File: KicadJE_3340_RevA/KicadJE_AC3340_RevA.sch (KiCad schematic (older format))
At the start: 125 parts, among them J101 RampOut1, J102 PulseOut2, J103 SawOut3, J104 In1.1, J105 In1.2, J106 In1.3, J107 SS_In2, J108 HS_In3, J109 FM_In4, J110 PWM_In5, J111 SineOut4, P101 HEADER_2x5_Doepfer, Q101 MMBT3906, Q102 UMX1N, SW101 Octave (3 state), U101 TL072, U102 TL072, U103 TL072, U104 AS3340, U105 L78L05_SOT89, U106 L79L05_SOT89, U107 TL072

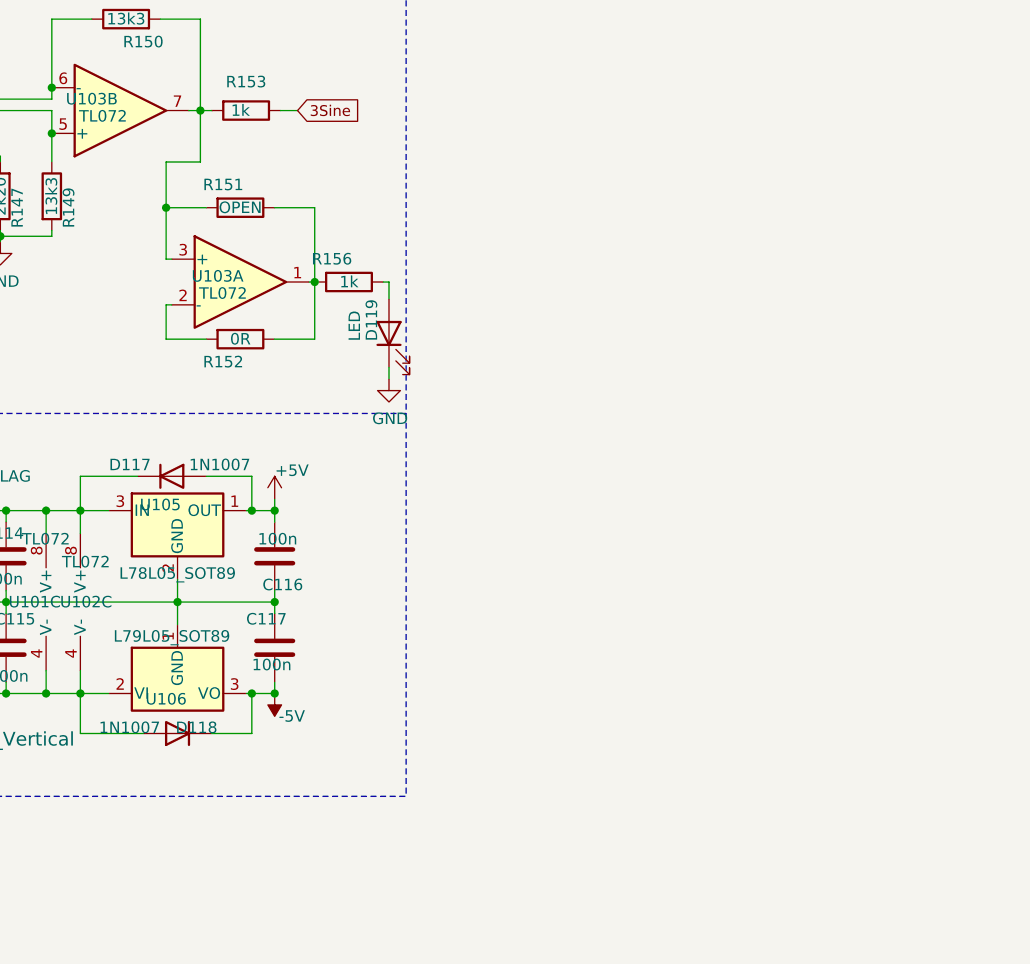
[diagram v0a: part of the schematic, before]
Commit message: Update KicadJE_AC3340_RevA.sch
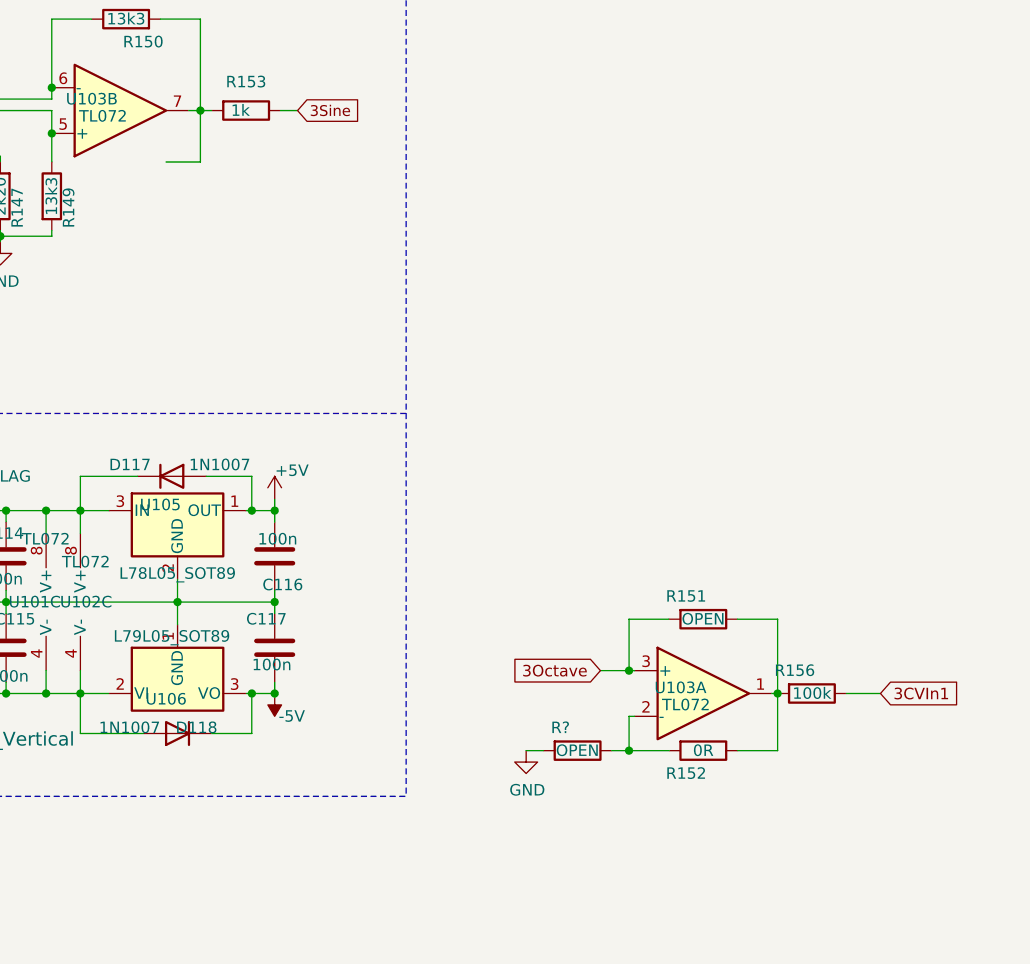
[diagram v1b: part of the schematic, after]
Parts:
- removed D119: LED, LED_SMD:LED_0805_2012Metric_Pad1.15x1.40mm_HandSolder, symbol Device:LED
- added R?: OPEN, Resistor_SMD:R_0805_2012Metric_Pad1.15x1.40mm_HandSolder, symbol Device:R
- R156: value 1k -> 100k
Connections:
- net 3CVIn1: now also R156.1
- net 3Octave: now also R151.2, U103.3 (+)
- net GND: now also R?.2
- net at R150.2, R153.2, U103.7: no longer R151.2, U103.3 (+)
- net at R152.2, U103.2 (-): now also R?.1
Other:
- moved on the sheet: R151, R152, R156, U103A
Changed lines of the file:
@@
 L Amplifier_Operational:TL072 U?
 U 1 1 614891B3
-P 7725 4275
+P 9750 6075
 AR Path="/5D99B81E/614891B3" Ref="U?"  Part="3"
 AR Path="/5D99B7BA/614891B3" Ref="U?"  Part="1"
@@
 AR Path="/5F49A670/614891B3" Ref="U?"  Part="1"
 AR Path="/614891B3" Ref="U103"  Part="1"
-F 0 "U103" H 7625 4300 50  0000 C CNN
-F 1 "TL072" H 7650 4225 50  0000 C CNN
-F 2 "AJ-Dropbox-Kicad:AJ_SO-8_5.3x6.2mm_P1.27mm" H 7725 4275 50  0001 C CNN
-F 3 "http://www.ti.com/lit/ds/symlink/tl071.pdf" H 7725 4275 50  0001 C CNN
-	1    7725 4275
+F 0 "U103" H 9650 6100 50  0000 C CNN
+F 1 "TL072" H 9675 6025 50  0000 C CNN
+F 2 "AJ-Dropbox-Kicad:AJ_SO-8_5.3x6.2mm_P1.27mm" H 9750 6075 50  0001 C CNN
+F 3 "http://www.ti.com/lit/ds/symlink/tl071.pdf" H 9750 6075 50  0001 C CNN
+	1    9750 6075
 	1    0    0    -1
 $EndComp
 Wire Wire Line
-	7425 4375 7400 4375
+	9450 6175 9425 6175
 Wire Wire Line
-	7400 4375 7400 4525
+	9425 6175 9425 6325
 Wire Wire Line
-	7400 4525 7575 4525
+	9425 6325 9600 6325
 Wire Wire Line
-	8050 4525 8050 4275
+	10075 6325 10075 6075
 Wire Wire Line
-	8050 4275 8025 4275
+	10075 6075 10050 6075
 $Comp
 L Device:R R156
 U 1 1 614891BF
-P 8200 4275
+P 10225 6075
 AR Path="/614891BF" Ref="R156"  Part="1"
 AR Path="/5C8C5FC0/614891BF" Ref="R?"  Part="1"
@@
 AR Path="/5E62ACA1/614891BF" Ref="R?"  Part="1"
 AR Path="/5F49A670/614891BF" Ref="R?"  Part="1"
-F 0 "R156" V 8100 4200 50  0000 C CNN
-F 1 "1k" V 8200 4275 50  0000 C CNN
-F 2 "Resistor_SMD:R_0805_2012Metric_Pad1.15x1.40mm_HandSolder" V 8130 4275 50  0001 C CNN
-F 3 "~" H 8200 4275 50  0001 C CNN
-	1    8200 4275
+F 0 "R156" V 10125 6000 50  0000 C CNN
+F 1 "100k" V 10225 6075 50  0000 C CNN
+F 2 "Resistor_SMD:R_0805_2012Metric_Pad1.15x1.40mm_HandSolder" V 10155 6075 50  0001 C CNN
+F 3 "~" H 10225 6075 50  0001 C CNN
+	1    10225 6075
 	0    1    1    0
 $EndComp
-Connection ~ 8050 4275
+Connection ~ 10075 6075
 Wire Wire Line
 	2400 1125 2325 1125
@@
 L Device:R R151
 U 1 1 61551447
-P 7725 3950
+P 9750 5750
 AR Path="/61551447" Ref="R151"  Part="1"
 AR Path="/5C8C5FC0/61551447" Ref="R?"  Part="1"
@@
 AR Path="/5E62ACA1/61551447" Ref="R?"  Part="1"
 AR Path="/5F49A670/61551447" Ref="R?"  Part="1"
-F 0 "R151" V 7625 3875 50  0000 C CNN
-F 1 "OPEN" V 7725 3950 50  0000 C CNN
-F 2 "Resistor_SMD:R_0805_2012Metric_Pad1.15x1.40mm_HandSolder" V 7655 3950 50  0001 C CNN
-F 3 "~" H 7725 3950 50  0001 C CNN
-	1    7725 3950
+F 0 "R151" V 9650 5675 50  0000 C CNN
+F 1 "OPEN" V 9750 5750 50  0000 C CNN
+F 2 "Resistor_SMD:R_0805_2012Metric_Pad1.15x1.40mm_HandSolder" V 9680 5750 50  0001 C CNN
+F 3 "~" H 9750 5750 50  0001 C CNN
+	1    9750 5750
 	0    1    1    0
 $EndComp
 Wire Wire Line
-	7400 4175 7400 3950
+	9425 5975 9425 5750
 Wire Wire Line
-	7400 3950 7575 3950
+	9425 5750 9600 5750
 Wire Wire Line
-	7400 4175 7425 4175
+	9425 5975 9450 5975
 Wire Wire Line
-	8050 4275 8050 3950
+	10075 6075 10075 5750
 Wire Wire Line
-	8050 3950 7875 3950
+	10075 5750 9900 5750
 $Comp
 L Envelope-cache-2018-08-04-13-00-04:GND #PWR0125
@@
 Wire Wire Line
 	7550 3750 7400 3750
-Wire Wire Line
-	7400 3750 7400 3950
-Connection ~ 7400 3950
 $Comp
 L Device:R R152
 U 1 1 616AB5FE
-P 7725 4525
+P 9750 6325
 AR Path="/616AB5FE" Ref="R152"  Part="1"
 AR Path="/5C8C5FC0/616AB5FE" Ref="R?"  Part="1"
@@
 AR Path="/5E62ACA1/616AB5FE" Ref="R?"  Part="1"
 AR Path="/5F49A670/616AB5FE" Ref="R?"  Part="1"
-F 0 "R152" V 7825 4450 50  0000 C CNN
-F 1 "0R" V 7725 4525 50  0000 C CNN
-F 2 "Resistor_SMD:R_0805_2012Metric_Pad1.15x1.40mm_HandSolder" V 7655 4525 50  0001 C CNN
-F 3 "~" H 7725 4525 50  0001 C CNN
-	1    7725 4525
+F 0 "R152" V 9850 6250 50  0000 C CNN
+F 1 "0R" V 9750 6325 50  0000 C CNN
+F 2 "Resistor_SMD:R_0805_2012Metric_Pad1.15x1.40mm_HandSolder" V 9680 6325 50  0001 C CNN
+F 3 "~" H 9750 6325 50  0001 C CNN
+	1    9750 6325
 	0    1    1    0
 $EndComp
 Wire Wire Line
-	7875 4525 8050 4525
+	9900 6325 10075 6325
+Text GLabel 10525 6075 2    50   Input ~ 0
+3CVIn1
+Wire Wire Line
+	10375 6075 10525 6075
+Text GLabel 9300 5975 0    50   Input ~ 0
+3Octave
+Wire Wire Line
+	9300 5975 9425 5975
+Connection ~ 9425 5975
 $Comp
-L Device:LED D?
-U 1 1 616ABD5F
-P 8375 4500
-AR Path="/5E4B0DD9/616ABD5F" Ref="D?"  Part="1"
-AR Path="/5E62ACA1/616ABD5F" Ref="D?"  Part="1"
-AR Path="/5F49A670/616ABD5F" Ref="D?"  Part="1"
-AR Path="/616ABD5F" Ref="D119"  Part="1"
-F 0 "D119" H 8525 4575 50  0000 R CNN
-F 1 "LED" H 8475 4650 50  0000 R CNN
-F 2 "LED_SMD:LED_0805_2012Metric_Pad1.15x1.40mm_HandSolder" H 8375 4500 50  0001 C CNN
-F 3 "~" H 8375 4500 50  0001 C CNN
-	1    8375 4500
-	0    -1   -1   0
+L Device:R R?
+U 1 1 5E78950E
+P 9200 6325
+AR Path="/5E78950E" Ref="R?"  Part="1"
+AR Path="/5C8C5FC0/5E78950E" Ref="R?"  Part="1"
+AR Path="/5CAAE8D3/5E78950E" Ref="R?"  Part="1"
+AR Path="/5E4B0DD9/5E78950E" Ref="R?"  Part="1"
+AR Path="/5E62ACA1/5E78950E" Ref="R?"  Part="1"
+AR Path="/5F49A670/5E78950E" Ref="R?"  Part="1"
+F 0 "R?" V 9100 6250 50  0000 C CNN
+F 1 "OPEN" V 9200 6325 50  0000 C CNN
+F 2 "Resistor_SMD:R_0805_2012Metric_Pad1.15x1.40mm_HandSolder" V 9130 6325 50  0001 C CNN
+F 3 "~" H 9200 6325 50  0001 C CNN
+	1    9200 6325
+	0    1    1    0
 $EndComp
 $Comp
-L Envelope-cache-2018-08-04-13-00-04:GND #PWR0142
-U 1 1 616AD7D0
-P 8375 4700
-AR Path="/616AD7D0" Ref="#PWR0142"  Part="1"
-AR Path="/5C8C5FC0/616AD7D0" Ref="#PWR?"  Part="1"
-AR Path="/5CAAE8D3/616AD7D0" Ref="#PWR?"  Part="1"
-AR Path="/5E4B0DD9/616AD7D0" Ref="#PWR?"  Part="1"
-AR Path="/5E62ACA1/616AD7D0" Ref="#PWR?"  Part="1"
-AR Path="/5F49A670/616AD7D0" Ref="#PWR?"  Part="1"
-F 0 "#PWR0142" H 8375 4450 50  0001 C CNN
-F 1 "GND" H 8380 4527 50  0000 C CNN
-F 2 "" H 8375 4700 50  0001 C CNN
-F 3 "" H 8375 4700 50  0001 C CNN
-	1    8375 4700
+L Envelope-cache-2018-08-04-13-00-04:GND #PWR?
+U 1 1 5E789A07
+P 8975 6325
+AR Path="/5E789A07" Ref="#PWR?"  Part="1"
+AR Path="/5C8C5FC0/5E789A07" Ref="#PWR?"  Part="1"
+AR Path="/5CAAE8D3/5E789A07" Ref="#PWR?"  Part="1"
+AR Path="/5E4B0DD9/5E789A07" Ref="#PWR?"  Part="1"
+AR Path="/5E62ACA1/5E789A07" Ref="#PWR?"  Part="1"
+AR Path="/5F49A670/5E789A07" Ref="#PWR?"  Part="1"
+F 0 "#PWR?" H 8975 6075 50  0001 C CNN
+F 1 "GND" H 8980 6152 50  0000 C CNN
+F 2 "" H 8975 6325 50  0001 C CNN
+F 3 "" H 8975 6325 50  0001 C CNN
+	1    8975 6325
 	1    0    0    -1
 $EndComp
 Wire Wire Line
-	8375 4700 8375 4650
+	8975 6325 9050 6325
 Wire Wire Line
-	8375 4275 8350 4275
-Wire Wire Line
-	8375 4350 8375 4275
+	9350 6325 9425 6325
+Connection ~ 9425 6325
 $EndSCHEMATC
